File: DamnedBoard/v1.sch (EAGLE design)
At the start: 15 parts, among them U1 EFM32ZG108, U2 MAX44009EDT+T21-0490D-M

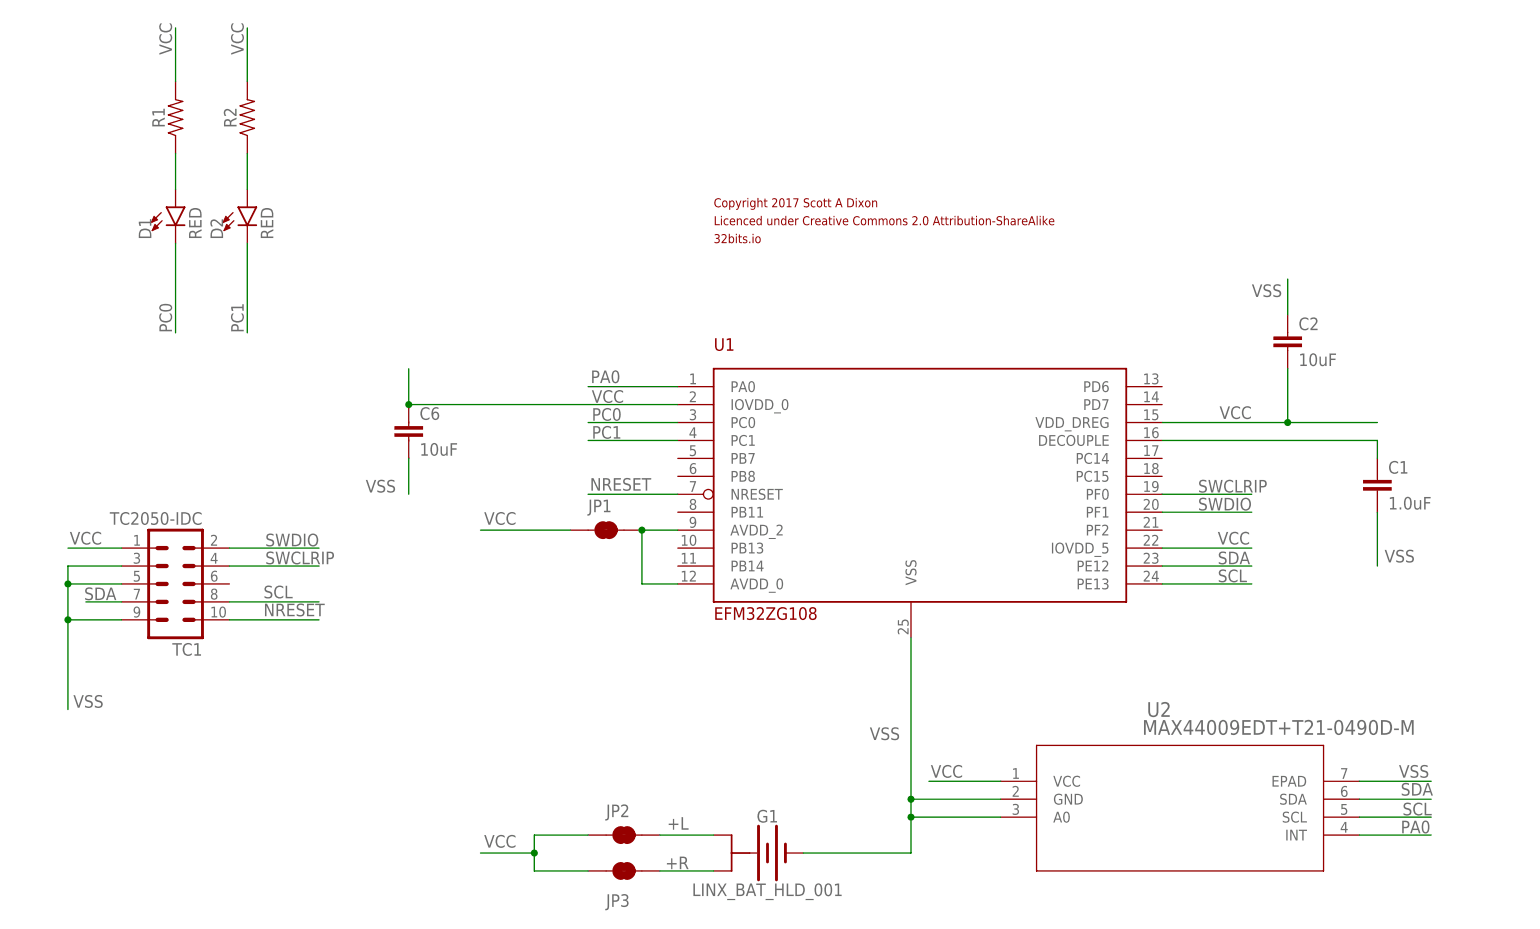
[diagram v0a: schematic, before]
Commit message: Candidate for manufacturing.
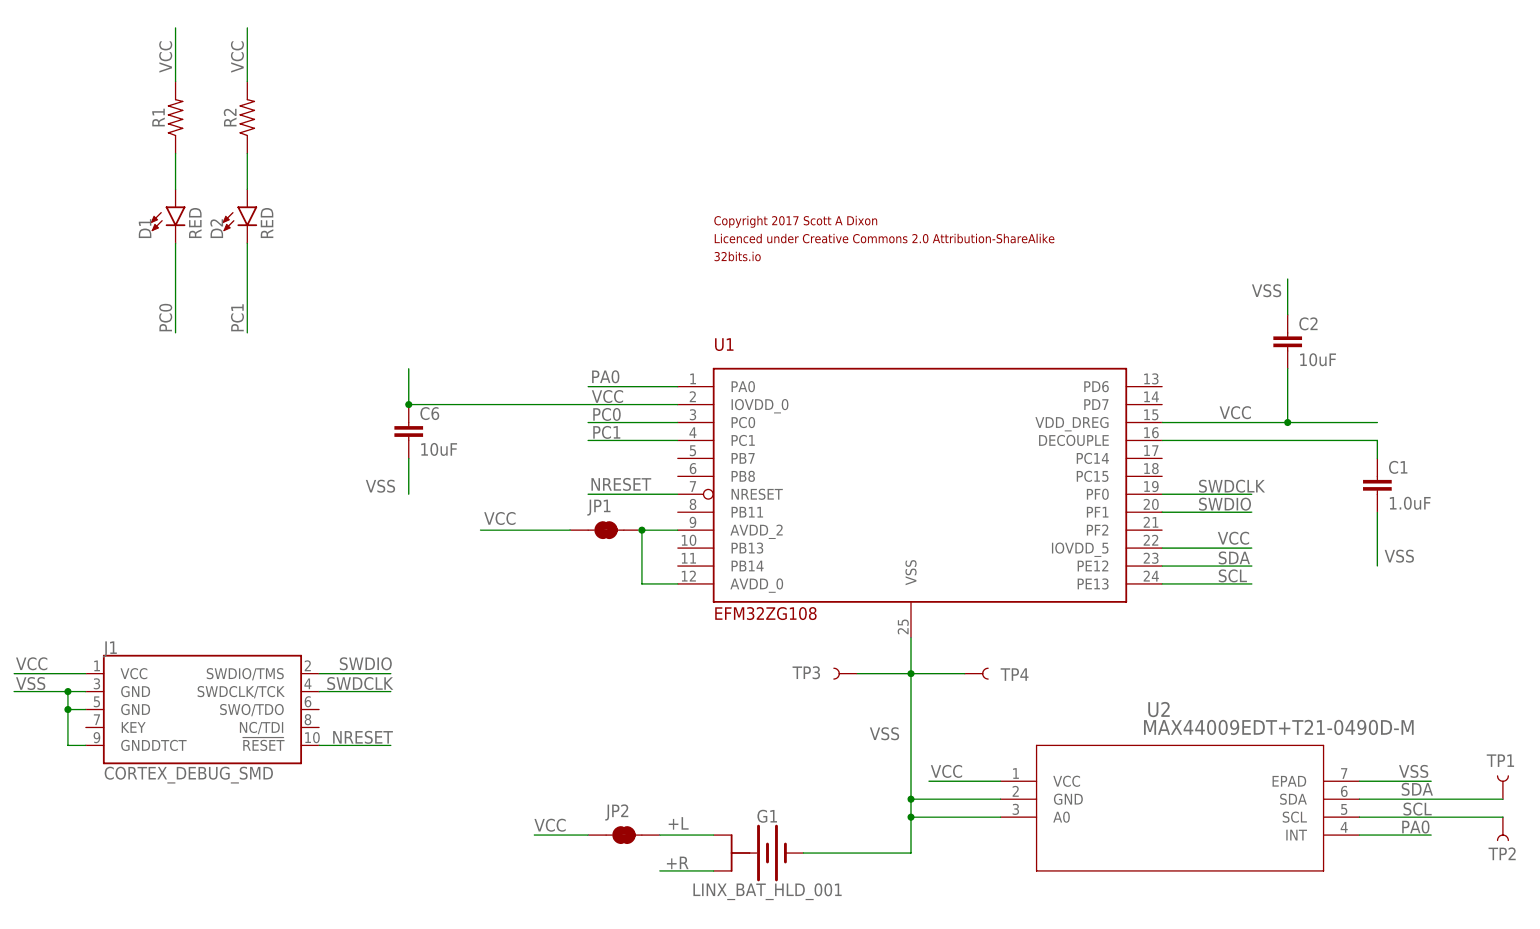
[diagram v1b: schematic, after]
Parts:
- removed JP3: JUMPER-SMT_2_NC_TRACE_NO-SILK, SparkFun-Jumpers:JUMPER-SMT_2_NC_TRACE_NO-SILK
- removed TC1: TC2050-IDC, TagConnect:TC2050-IDC
- added J1: CORTEX_DEBUG_SMD, SparkFun-Connectors:CORTEX_DEBUG_SMD
- added TP1, TP2, TP3, TP4: TEST-POINT3, SparkFun-Connectors:TEST-POINT3
- U$1: value DAMNED -> COPYRIGHT; device boneyard:DAMNED -> boneyard:COPYRIGHT
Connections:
- net N$4 renamed AVDD
- removed net SWCLRIP: TC1.4, U1.PF0
- new net SWDCLK: J1.SWDCLK/TCK, U1.PF0
- net +R: no longer JP3.2
- net NRESET: now also J1.!RESET; no longer TC1.10
- net SCL: now also TP2.1; no longer TC1.8
- net SDA: now also TP1.1; no longer TC1.7
- net SWDIO: now also J1.SWDIO/TMS; no longer TC1.2
- net VCC: now also J1.VCC; no longer JP3.1, TC1.1
- net VSS: now also J1.GND@3, J1.GND@5, J1.GNDDTCT, TP3.1, TP4.1; no longer TC1.3, TC1.5, TC1.9
